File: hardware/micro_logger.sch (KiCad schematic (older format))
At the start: 26 parts, among them J4 power, J5 DM3AT-SF-PEJM5, SW2 SW_Push, U1 MIC5205-3.3, U2 TLV70218_SOT23-5, U4 ICM-20948, U5 PCA9306

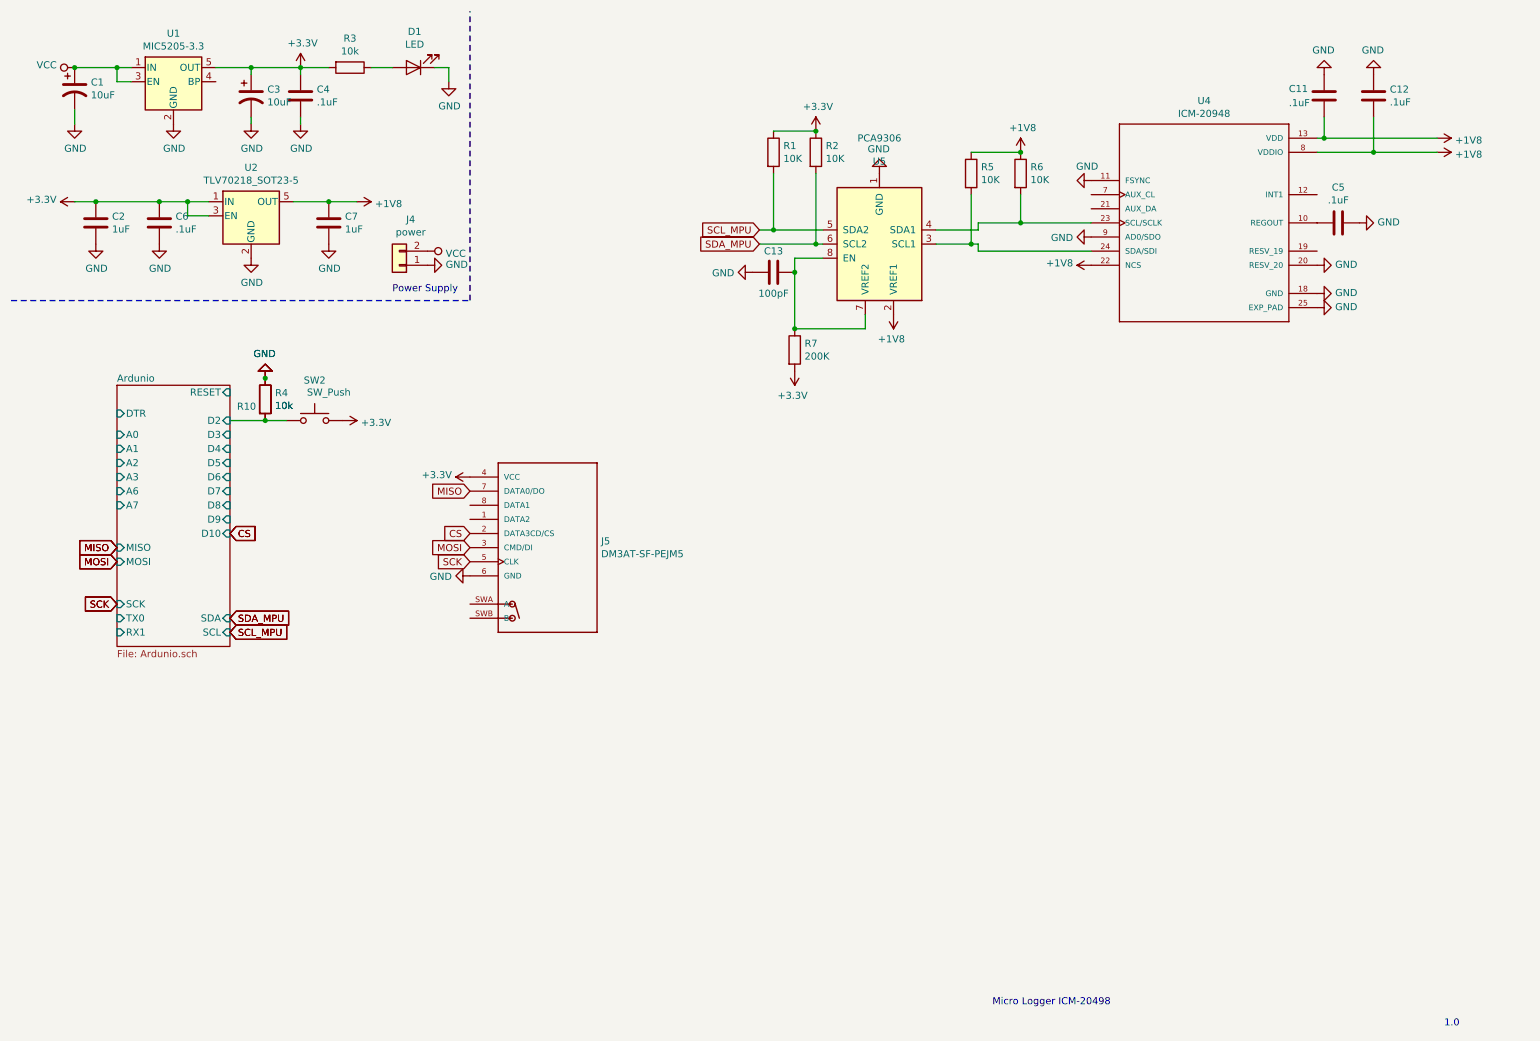
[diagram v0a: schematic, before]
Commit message: updated schematic
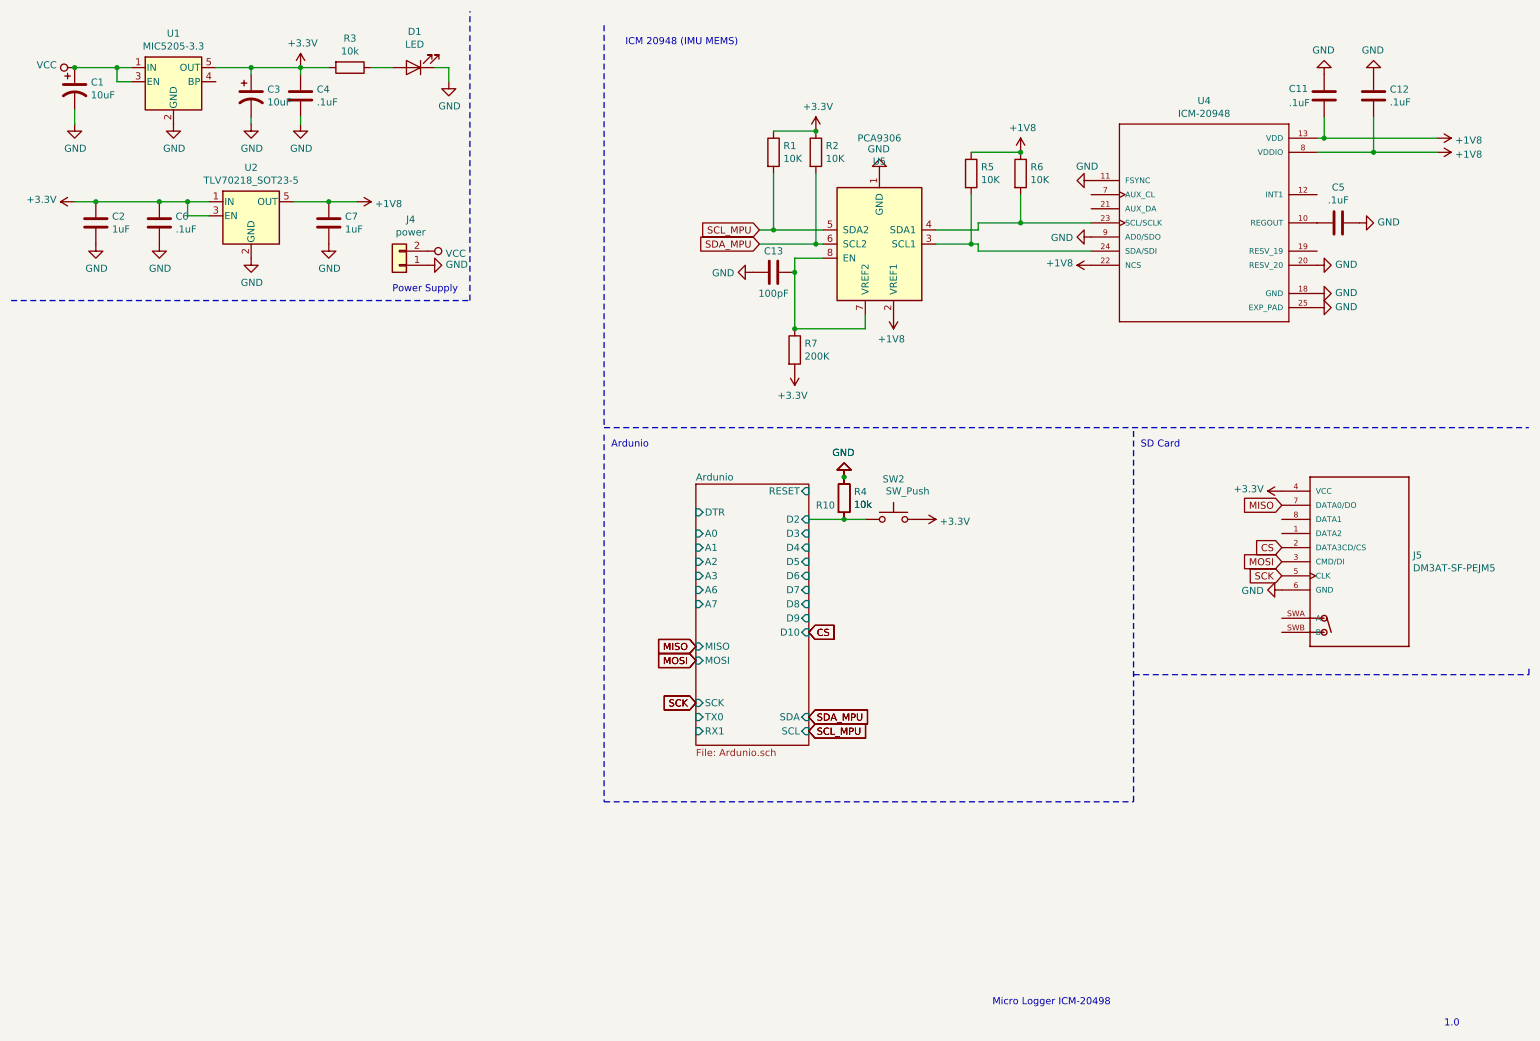
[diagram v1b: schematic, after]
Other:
- note added: "Ardunio\n"
- note added: "ICM 20948 (IMU MEMS)\n"
- note added: "SD Card\n"
- moved on the sheet: J5, R10, R4, SW2
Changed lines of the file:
@@
 $EndDescr
 $Sheet
-S 1200 3100 800  1850
+S 5300 3800 800  1850
 U 5B10C25E
 F0 "Ardunio" 50
 F1 "Ardunio.sch" 50
-F2 "DTR" I L 1200 3300 50
-F3 "A0" I L 1200 3450 50
-F4 "A1" I L 1200 3550 50
-F5 "A2" I L 1200 3650 50
-F6 "A3" I L 1200 3750 50
-F7 "SDA" I R 2000 4750 50
-F8 "SCL" I R 2000 4850 50
-F9 "TX0" I L 1200 4750 50
-F10 "RX1" I L 1200 4850 50
-F11 "D2" I R 2000 3350 50
-F12 "D3" I R 2000 3450 50
-F13 "D4" I R 2000 3550 50
-F14 "D5" I R 2000 3650 50
-F15 "D6" I R 2000 3750 50
-F16 "D7" I R 2000 3850 50
-F17 "D9" I R 2000 4050 50
-F18 "D8" I R 2000 3950 50
-F19 "D10" I R 2000 4150 50
-F20 "MOSI" I L 1200 4350 50
-F21 "MISO" I L 1200 4250 50
-F22 "SCK" I L 1200 4650 50
-F23 "A6" I L 1200 3850 50
-F24 "A7" I L 1200 3950 50
-F25 "RESET" I R 2000 3150 50
+F2 "DTR" I L 5300 4000 50
+F3 "A0" I L 5300 4150 50
+F4 "A1" I L 5300 4250 50
+F5 "A2" I L 5300 4350 50
+F6 "A3" I L 5300 4450 50
+F7 "SDA" I R 6100 5450 50
+F8 "SCL" I R 6100 5550 50
+F9 "TX0" I L 5300 5450 50
+F10 "RX1" I L 5300 5550 50
+F11 "D2" I R 6100 4050 50
+F12 "D3" I R 6100 4150 50
+F13 "D4" I R 6100 4250 50
+F14 "D5" I R 6100 4350 50
+F15 "D6" I R 6100 4450 50
+F16 "D7" I R 6100 4550 50
+F17 "D9" I R 6100 4750 50
+F18 "D8" I R 6100 4650 50
+F19 "D10" I R 6100 4850 50
+F20 "MOSI" I L 5300 5050 50
+F21 "MISO" I L 5300 4950 50
+F22 "SCK" I L 5300 5350 50
+F23 "A6" I L 5300 4550 50
+F24 "A7" I L 5300 4650 50
+F25 "RESET" I R 6100 3850 50
 $EndSheet
 $Comp
@@
 L SD:DM3AT-SF-PEJM5 J5
 U 1 1 5B292A17
-P 3900 4250
-F 0 "J5" H 4629 4296 50  0000 L CNN
-F 1 "DM3AT-SF-PEJM5" H 4629 4205 50  0000 L CNN
-F 2 "components:HRS_DM3AT-SF-PEJM5" H 3900 4250 50  0001 L BNN
-F 3 "None" H 3900 4250 50  0001 L BNN
-F 4 "Hirose" H 3900 4250 50  0001 L BNN "Field4"
-F 5 "DM3AT-SF-PEJM5" H 3900 4250 50  0001 L BNN "Field5"
-F 6 "Warning" H 3900 4250 50  0001 L BNN "Field6"
-F 7 "2.58 USD" H 3900 4250 50  0001 L BNN "Field7"
-F 8 "DM3 RA SMT microSD memory card push/push" H 3900 4250 50  0001 L BNN "Field8"
-	1    3900 4250
+P 9650 4350
+F 0 "J5" H 10379 4396 50  0000 L CNN
+F 1 "DM3AT-SF-PEJM5" H 10379 4305 50  0000 L CNN
+F 2 "components:HRS_DM3AT-SF-PEJM5" H 9650 4350 50  0001 L BNN
+F 3 "None" H 9650 4350 50  0001 L BNN
+F 4 "Hirose" H 9650 4350 50  0001 L BNN "Field4"
+F 5 "DM3AT-SF-PEJM5" H 9650 4350 50  0001 L BNN "Field5"
+F 6 "Warning" H 9650 4350 50  0001 L BNN "Field6"
+F 7 "2.58 USD" H 9650 4350 50  0001 L BNN "Field7"
+F 8 "DM3 RA SMT microSD memory card push/push" H 9650 4350 50  0001 L BNN "Field8"
+	1    9650 4350
 	1    0    0    -1
 $EndComp
@@
 L power:+3.3V #PWR0116
 U 1 1 5B292D16
-P 3700 3750
-F 0 "#PWR0116" H 3700 3600 50  0001 C CNN
-F 1 "+3.3V" V 3715 3878 50  0000 L CNN
-F 2 "" H 3700 3750 50  0001 C CNN
-F 3 "" H 3700 3750 50  0001 C CNN
-	1    3700 3750
+P 9450 3850
+F 0 "#PWR0116" H 9450 3700 50  0001 C CNN
+F 1 "+3.3V" V 9465 3978 50  0000 L CNN
+F 2 "" H 9450 3850 50  0001 C CNN
+F 3 "" H 9450 3850 50  0001 C CNN
+	1    9450 3850
 	0    -1   -1   0
 $EndComp
-Text GLabel 3700 4150 0    50   Input ~ 0
+Text GLabel 9450 4250 0    50   Input ~ 0
 CS
-Text GLabel 2000 4150 2    50   Input ~ 0
+Text GLabel 6100 4850 2    50   Input ~ 0
 CS
-Text GLabel 3700 4350 0    50   Input ~ 0
+Text GLabel 9450 4450 0    50   Input ~ 0
 SCK
-Text GLabel 1200 4650 0    50   Input ~ 0
+Text GLabel 5300 5350 0    50   Input ~ 0
 SCK
 $Comp
 L power:GND #PWR0117
 U 1 1 5B293C50
-P 3700 4450
-F 0 "#PWR0117" H 3700 4200 50  0001 C CNN
-F 1 "GND" V 3705 4322 50  0000 R CNN
-F 2 "" H 3700 4450 50  0001 C CNN
-F 3 "" H 3700 4450 50  0001 C CNN
-	1    3700 4450
-	0    1    1    0
-$EndComp
-Text GLabel 1200 4350 0    50   Input ~ 0
+P 9450 4550
+F 0 "#PWR0117" H 9450 4300 50  0001 C CNN
+F 1 "GND" V 9455 4422 50  0000 R CNN
+F 2 "" H 9450 4550 50  0001 C CNN
+F 3 "" H 9450 4550 50  0001 C CNN
+	1    9450 4550
+	0    1    1    0
+$EndComp
+Text GLabel 5300 5050 0    50   Input ~ 0
 MOSI
-Text GLabel 3700 4250 0    50   Input ~ 0
+Text GLabel 9450 4350 0    50   Input ~ 0
 MOSI
-Text GLabel 1200 4250 0    50   Input ~ 0
+Text GLabel 5300 4950 0    50   Input ~ 0
 MISO
-Text GLabel 3700 3850 0    50   Input ~ 0
+Text GLabel 9450 3950 0    50   Input ~ 0
 MISO
 $Comp
 L Switch:SW_Push SW2
 U 1 1 5BB13284
-P 2600 3350
-F 0 "SW2" H 2600 3635 50  0000 C CNN
-F 1 "SW_Push" H 2700 3550 50  0000 C CNN
-F 2 "Buttons_Switches_SMD:SW_SPST_B3U-1000P" H 2600 3550 50  0001 C CNN
-F 3 "" H 2600 3550 50  0001 C CNN
-	1    2600 3350
+P 6700 4050
+F 0 "SW2" H 6700 4335 50  0000 C CNN
+F 1 "SW_Push" H 6800 4250 50  0000 C CNN
+F 2 "Buttons_Switches_SMD:SW_SPST_B3U-1000P" H 6700 4250 50  0001 C CNN
+F 3 "" H 6700 4250 50  0001 C CNN
+	1    6700 4050
 	1    0    0    -1
 $EndComp
@@
 L power:+3.3V #PWR0108
 U 1 1 5BB13765
-P 2800 3350
-F 0 "#PWR0108" H 2800 3200 50  0001 C CNN
-F 1 "+3.3V" V 2815 3478 50  0000 L CNN
-F 2 "" H 2800 3350 50  0001 C CNN
-F 3 "" H 2800 3350 50  0001 C CNN
-	1    2800 3350
-	0    1    1    0
-$EndComp
-Wire Wire Line
-	2000 3350 2250 3350
+P 6900 4050
+F 0 "#PWR0108" H 6900 3900 50  0001 C CNN
+F 1 "+3.3V" V 6915 4178 50  0000 L CNN
+F 2 "" H 6900 4050 50  0001 C CNN
+F 3 "" H 6900 4050 50  0001 C CNN
+	1    6900 4050
+	0    1    1    0
+$EndComp
+Wire Wire Line
+	6100 4050 6350 4050
 $Comp
 L Device:R R4
 U 1 1 5BB13EB6
-P 2250 3200
-F 0 "R4" H 2320 3246 50  0000 L CNN
-F 1 "10k" H 2320 3155 50  0000 L CNN
-F 2 "Resistor_SMD:R_0805_2012Metric" V 2180 3200 50  0001 C CNN
-F 3 "~" H 2250 3200 50  0001 C CNN
-	1    2250 3200
-	1    0    0    -1
-$EndComp
-Connection ~ 2250 3350
+P 6350 3900
+F 0 "R4" H 6420 3946 50  0000 L CNN
+F 1 "10k" H 6420 3855 50  0000 L CNN
+F 2 "Resistor_SMD:R_0805_2012Metric" V 6280 3900 50  0001 C CNN
+F 3 "~" H 6350 3900 50  0001 C CNN
+	1    6350 3900
+	1    0    0    -1
+$EndComp
+Connection ~ 6350 4050
 $Comp
 L power:GND #PWR0109
 U 1 1 5BB13F64
-P 2250 3050
-F 0 "#PWR0109" H 2250 2800 50  0001 C CNN
-F 1 "GND" H 2255 2877 50  0000 C CNN
-F 2 "" H 2250 3050 50  0001 C CNN
-F 3 "" H 2250 3050 50  0001 C CNN
-	1    2250 3050
+P 6350 3750
+F 0 "#PWR0109" H 6350 3500 50  0001 C CNN
+F 1 "GND" H 6355 3577 50  0000 C CNN
+F 2 "" H 6350 3750 50  0001 C CNN
+F 3 "" H 6350 3750 50  0001 C CNN
+	1    6350 3750
 	-1   0    0    1
 $EndComp
 Wire Wire Line
-	2250 3350 2400 3350
+	6350 4050 6500 4050
 Connection ~ 900  850
 $Comp
@@
 	0    -1   -1   0
 $EndComp
-Text GLabel 2000 4850 2    50   Input ~ 0
+Text GLabel 6100 5550 2    50   Input ~ 0
 SCL_MPU
-Text GLabel 2000 4750 2    50   Input ~ 0
+Text GLabel 6100 5450 2    50   Input ~ 0
 SDA_MPU
 $Comp
@@
 Text Notes 3150 2450 0    50   ~ 0
 Power Supply\n
-Text GLabel 2000 4150 2    50   Input ~ 0
+Text GLabel 6100 4850 2    50   Input ~ 0
 CS
-Text GLabel 1200 4650 0    50   Input ~ 0
+Text GLabel 5300 5350 0    50   Input ~ 0
 SCK
-Text GLabel 1200 4350 0    50   Input ~ 0
+Text GLabel 5300 5050 0    50   Input ~ 0
 MOSI
-Text GLabel 1200 4250 0    50   Input ~ 0
+Text GLabel 5300 4950 0    50   Input ~ 0
 MISO
 $Comp
 L Device:R R10
 U 1 1 5BF0C120
-P 2250 3200
-F 0 "R10" H 2050 3150 50  0000 L CNN
-F 1 "10k" H 2320 3155 50  0000 L CNN
-F 2 "Resistor_SMD:R_0805_2012Metric" V 2180 3200 50  0001 C CNN
-F 3 "~" H 2250 3200 50  0001 C CNN
-	1    2250 3200
+P 6350 3900
+F 0 "R10" H 6150 3850 50  0000 L CNN
+F 1 "10k" H 6420 3855 50  0000 L CNN
+F 2 "Resistor_SMD:R_0805_2012Metric" V 6280 3900 50  0001 C CNN
+F 3 "~" H 6350 3900 50  0001 C CNN
+	1    6350 3900
 	1    0    0    -1
 $EndComp
@@
 L power:GND #PWR0133
 U 1 1 5BF0C12B
-P 2250 3050
-F 0 "#PWR0133" H 2250 2800 50  0001 C CNN
-F 1 "GND" H 2255 2877 50  0000 C CNN
-F 2 "" H 2250 3050 50  0001 C CNN
-F 3 "" H 2250 3050 50  0001 C CNN
-	1    2250 3050
+P 6350 3750
+F 0 "#PWR0133" H 6350 3500 50  0001 C CNN
+F 1 "GND" H 6355 3577 50  0000 C CNN
+F 2 "" H 6350 3750 50  0001 C CNN
+F 3 "" H 6350 3750 50  0001 C CNN
+	1    6350 3750
 	-1   0    0    1
 $EndComp
-Text GLabel 2000 4850 2    50   Input ~ 0
+Text GLabel 6100 5550 2    50   Input ~ 0
 SCL_MPU
-Text GLabel 2000 4750 2    50   Input ~ 0
+Text GLabel 6100 5450 2    50   Input ~ 0
 SDA_MPU
-Connection ~ 2250 3050
+Connection ~ 6350 3750
 Text Notes 10600 7650 0    50   ~ 0
 1.0\n
+Wire Notes Line
+	4650 550  4650 3400
+Wire Notes Line
+	4650 3400 11200 3400
+Text Notes 4800 700  0    50   ~ 0
+ICM 20948 (IMU MEMS)\n
+Wire Notes Line
+	4650 3450 4650 6050
+Wire Notes Line
+	11200 5150 11200 5100
+Wire Notes Line
+	4650 6050 8400 6050
 Text Notes 7400 7500 0    50   ~ 0
 Micro Logger ICM-20498\n
+Text Notes 8450 3550 0    50   ~ 0
+SD Card\n
+Wire Notes Line
+	8400 5150 11200 5150
+Wire Notes Line
+	8400 6050 8400 3400
+Text Notes 4700 3550 0    50   ~ 0
+Ardunio\n
 $EndSCHEMATC
